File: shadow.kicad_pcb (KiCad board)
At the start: 2 copper layers, 69.8 x 78.7 mm, 100 parts, among them IC2 XB8089D, J1 USB_C_Receptacle, SW1 SW_Push, SW2 SW_Push, SW3 SW_SPST, U1 TCA9548APWR, U2 TCA9548APWR, U3 BQ24092DGQR, U4 TPS61085DGKR, U5 TPS259621DDAT

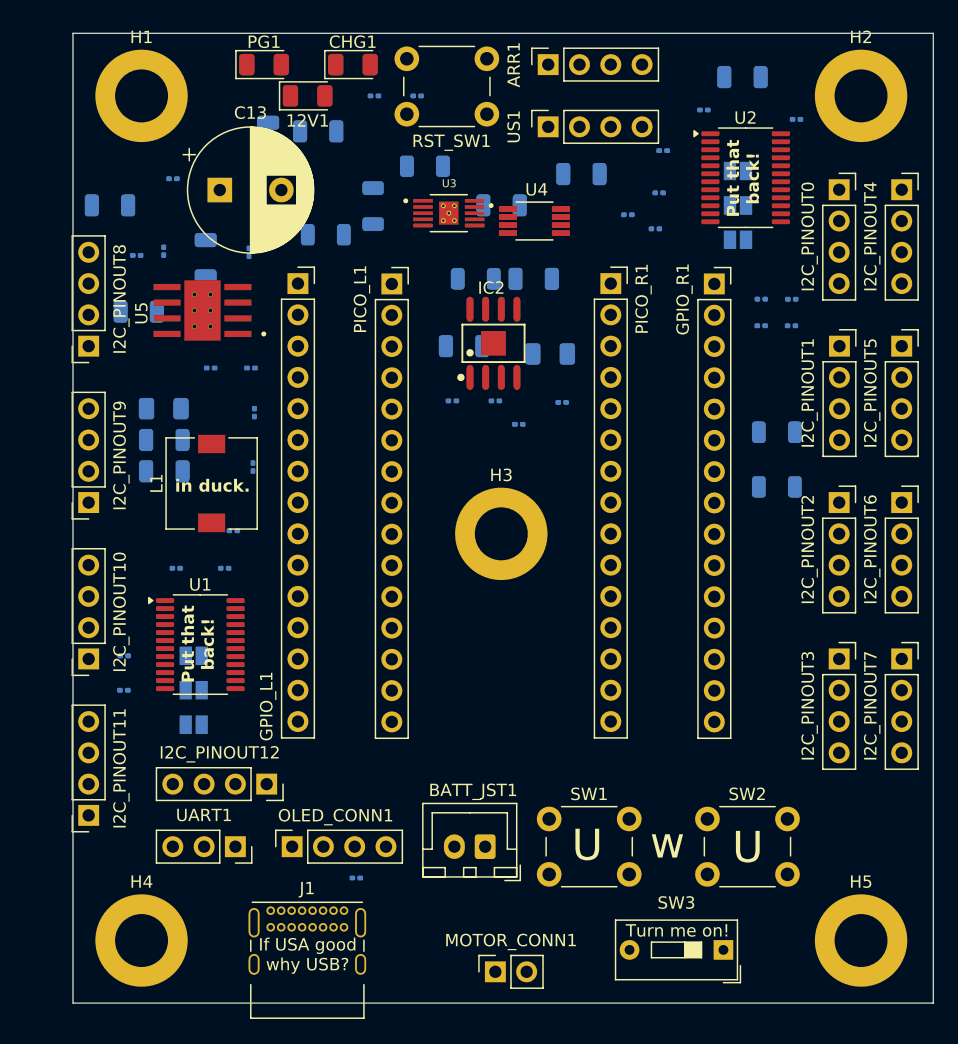
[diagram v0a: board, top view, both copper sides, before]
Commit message: fix some stuff and retrace
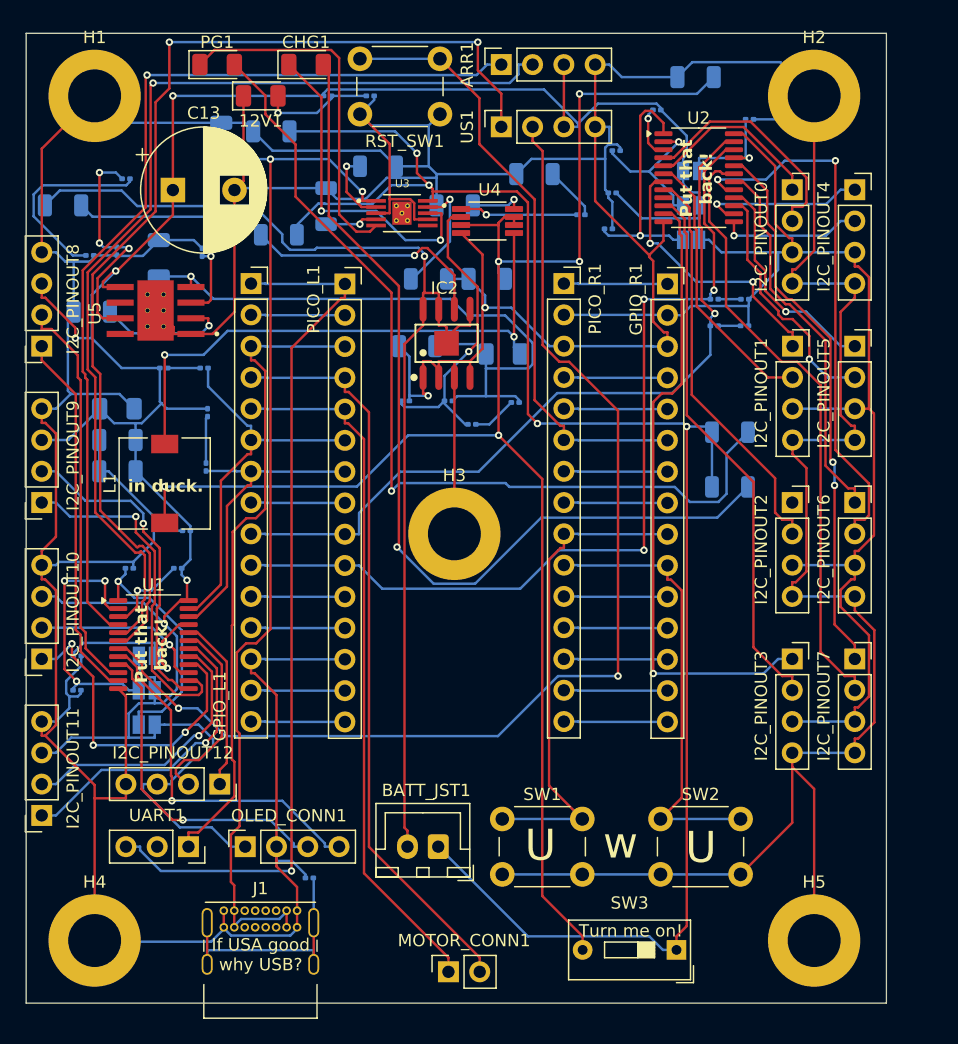
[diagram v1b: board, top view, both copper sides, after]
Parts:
- moved R3 3.81 mm to (125.6, 78.1)
- moved 12V1 3.81 mm to (113.8, 53.3)
- moved ARR1 3.81 mm to (133.3, 50.8)
- moved BATT_JST1 3.81 mm to (128.2, 114.3)
- moved C1 3.81 mm to (136.0, 59.7)
- moved C10 3.81 mm to (100.1, 70.9)
- moved C11 3.81 mm to (102.2, 81.3)
- moved C12 3.81 mm to (102.2, 83.8)
- moved C14 3.81 mm to (107.8, 88.6)
- moved C15 3.81 mm to (142.4, 61.2)
- moved C2 3.81 mm to (129.6, 62.2)
- moved C4 3.81 mm to (126.5, 73.7)
- moved C5 3.81 mm to (149.1, 51.8)
- moved C7 3.81 mm to (97.8, 62.2)
- moved C8 3.81 mm to (110.6, 57.0)
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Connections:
- GPIO_R1 pad 1: /GPIO29 -> /GPIO15
- GPIO_R1 pad 10: /GPIO20 -> /GPIO24
- GPIO_R1 pad 11: /GPIO19 -> /GPIO25
- GPIO_R1 pad 12: /GPIO18 -> /GPIO26
- GPIO_R1 pad 13: GND -> /GPIO27
- GPIO_R1 pad 14: VCC -> /GPIO28
- GPIO_R1 pad 15: /GPIO15 -> /GPIO29
- GPIO_R1 pad 2: /GPIO28 -> VCC
- GPIO_R1 pad 3: /GPIO27 -> GND
- GPIO_R1 pad 4: /GPIO26 -> /GPIO18
- GPIO_R1 pad 5: /GPIO25 -> /GPIO19
- GPIO_R1 pad 6: /GPIO24 -> /GPIO20
- GPIO_R1 pad 7: /GPIO23 -> /GPIO21
- GPIO_R1 pad 9: /GPIO21 -> /GPIO23
- PICO_R1 pad 1: /GPIO29 -> /GPIO15
- PICO_R1 pad 10: /GPIO20 -> /GPIO24
- PICO_R1 pad 11: /GPIO19 -> /GPIO25
- PICO_R1 pad 12: /GPIO18 -> /GPIO26
- PICO_R1 pad 13: GND -> /GPIO27
- PICO_R1 pad 14: VCC -> /GPIO28
- PICO_R1 pad 15: /GPIO15 -> /GPIO29
- PICO_R1 pad 2: /GPIO28 -> VCC
- PICO_R1 pad 3: /GPIO27 -> GND
- PICO_R1 pad 4: /GPIO26 -> /GPIO18
- PICO_R1 pad 5: /GPIO25 -> /GPIO19
- PICO_R1 pad 6: /GPIO24 -> /GPIO20
- PICO_R1 pad 7: /GPIO23 -> /GPIO21
- PICO_R1 pad 9: /GPIO21 -> /GPIO23
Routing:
- net GND: track 0.00 -> 565.2 mm, vias 0 -> 2
- net VCC: track 0.00 -> 315.7 mm, vias 0 -> 5
- net /battery/BAT+: track 0.00 -> 139.7 mm, vias 0 -> 4
- net Net-(SW3-B): track 0.00 -> 132.1 mm, vias 0 -> 5
- net /US_SCL: track 0.00 -> 93.8 mm, vias 0 -> 2
- net /battery/BAT-: track 0.00 -> 92.4 mm, vias 0 -> 1
- net /US_SDA: track 0.00 -> 87.7 mm, vias 0 -> 2
- net Net-(U3-IN): track 0.00 -> 85.2 mm, vias 0 -> 2
- net /SENSOR_SCL: track 0.00 -> 82.4 mm, vias 0 -> 1
- net /SENSOR_SDA: track 0.00 -> 77.5 mm, vias 0 -> 1
- net Net-(CHG1-A): track 0.00 -> 74.8 mm, vias 0 -> 1
- net Net-(PG1-A): track 0.00 -> 74.0 mm, vias 0 -> 1
- net /GPIO9: track 0.00 -> 73.7 mm, vias 0 -> 3
- net /GPIO0: track 0.00 -> 71.7 mm, vias 0 -> 1
- net /GPIO8: track 0.00 -> 63.9 mm, vias 0 -> 1
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
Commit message: v0.0.1
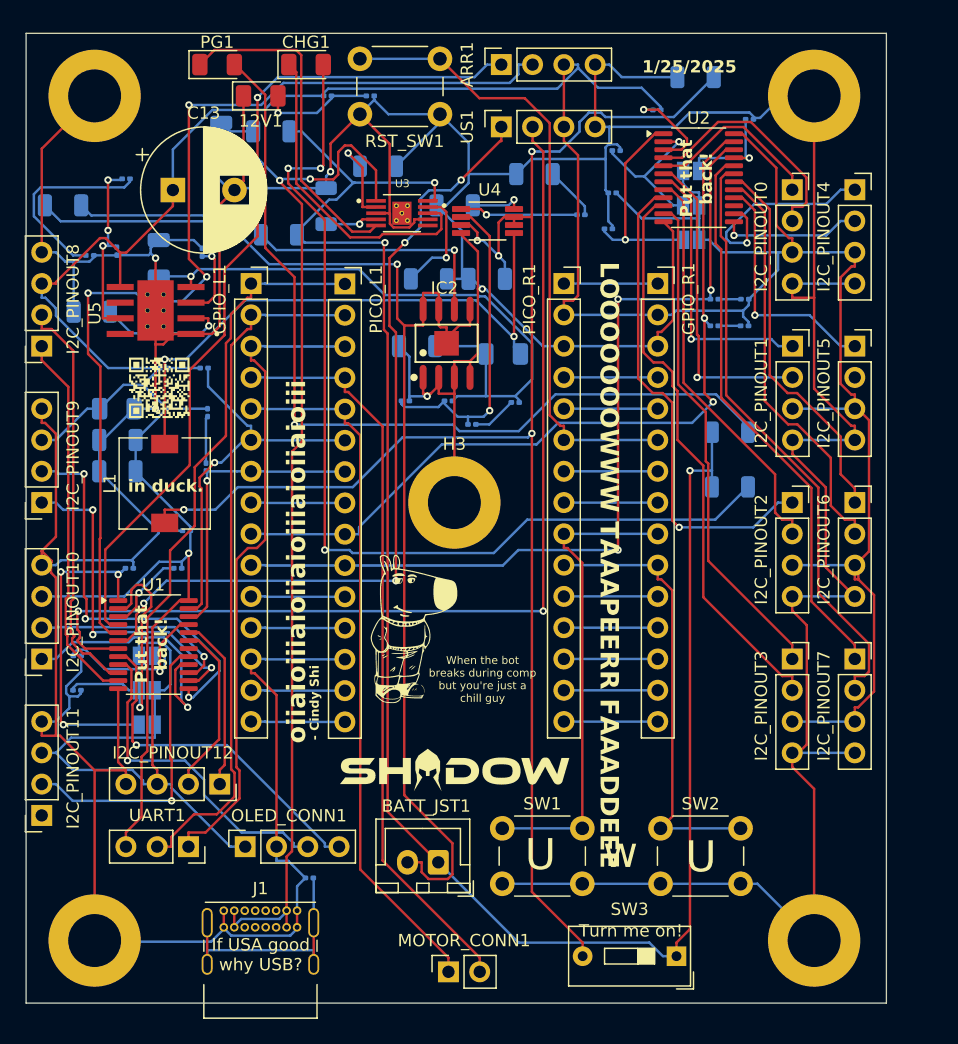
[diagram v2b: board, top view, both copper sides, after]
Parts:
- added G***: LOGO, LOGO, F.Cu at (127.0, 96.5)
- moved H3 2.54 mm to (129.5, 86.4)
- moved BATT_JST1 1.27 mm to (128.2, 115.6)
- moved GPIO_R1 0.79 mm to (146.1, 68.6)
- moved SW1 0.76 mm to (133.4, 112.8)
- moved SW2 0.76 mm to (146.3, 112.8)
- moved SW3 0.51 mm to (147.6, 123.2)
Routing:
- net /GPIO1: track 7.63 -> 56.1 mm
- net /I2C_PINOUT2/SCL: track 0.00 -> 39.9 mm, vias 0 -> 1
- net GND: track 565.2 -> 535.6 mm, vias 2 -> 5
- net /I2C_PINOUT11/SCL: track 25.1 -> 0.00 mm, vias 1 -> 0
- net /US_SDA: track 87.7 -> 67.5 mm, vias 2 -> 4
- net /I2C_PINOUT5/SDA: track 20.1 -> 0.00 mm, vias 1 -> 0
- net VCC: track 315.7 -> 330.3 mm, vias 5 -> 1
- net /GPIO0: track 71.7 -> 57.7 mm, vias 1 -> 0
- net /I2C_PINOUT6/SDA: track 44.3 -> 33.3 mm, vias 2 -> 0
- net /I2C_PINOUT3/SCL: track 51.6 -> 40.9 mm, vias 1 -> 0
- net /battery/BAT+: track 139.7 -> 150.1 mm, vias 4 -> 3
- net /US_SCL: track 93.8 -> 83.6 mm
- net /battery/BAT-: track 92.4 -> 100.6 mm
- net /SENSOR_SDA: track 77.5 -> 69.6 mm
- net /I2C_PINOUT9/SDA: track 26.1 -> 32.6 mm, vias 1 -> 3
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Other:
- board text added: "- Cindy Shi"
- board text added: "1/25/2025"
- board text added: "Designed & Developed by: Evan Yu Logo & Backseating: Aaron Huang"
- board text added: "LOOOOOOOWWW TAAAPEERR FAAADDEEE"
- board text added: "When the bot breaks during comp but you're just a chill guy"
- board text added: "oiiaioiiiaioiiaioiiiaioiiaioiii"
- board text added: "v0.0.1 ymci.ca/shadow"

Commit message: finish pcb
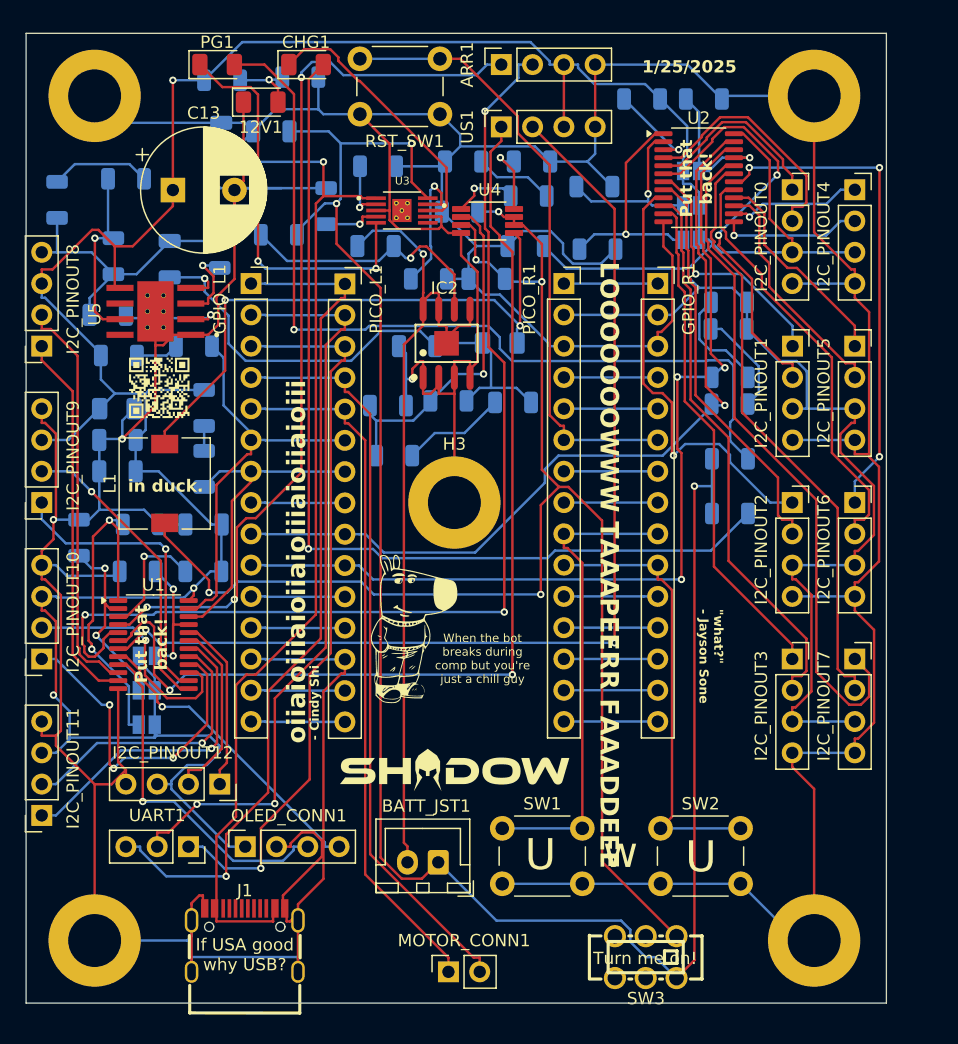
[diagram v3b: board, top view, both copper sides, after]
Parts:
- removed R30: 0k, Resistor_SMD:R_0201_0603Metric
- C14, C15: footprint Capacitor_SMD:C_0201_0603Metric -> Capacitor_SMD:C_1206_3216Metric
- J1: footprint Connector_USB:USB_C_Receptacle_GCT_USB4085 -> USB_C:TYPE-C-SMD_20009-UCAF001-X
- R1, R11, R12, R13, R14, R15, R16, R17, R18, R19, R2, R20, R21, R22, R23, R24, R25, R26, R27, R28, R29, R3, R31, R32, R33, R34, R4: footprint Resistor_SMD:R_0201_0603Metric -> Resistor_SMD:R_1206_3216Metric
- SW3: value SW_SPST -> ~; footprint Button_Switch_THT:SW_DIP_SPSTx01_Slide_9.78x4.72mm_W7.62mm_P2.54mm -> Switch:SW-TH_K3-2235D-F1
- moved C7 25.6 mm to (123.1, 65.5)
- moved C5 22.0 mm to (130.0, 62.7)
- moved R21 12.4 mm to (99.1, 89.2), turned to -90 degrees
- moved R14 8.65 mm to (110.7, 52.1)
- moved R22 8.43 mm to (103.8, 91.9), turned to 0 degrees
- moved C15 8.24 mm to (135.3, 65.5)
- moved C2 7.21 mm to (135.8, 58.7), turned to 0 degrees
- moved R1 6.80 mm to (124.7, 82.5)
- moved R32 6.48 mm to (151.9, 78.4)
- moved R34 6.48 mm to (151.9, 76.2)
- moved C1 5.88 mm to (130.3, 58.7)
- moved R15 5.88 mm to (117.0, 51.8)
- moved R13 5.23 mm to (97.3, 61.8), turned to 90 degrees
- moved R4 4.51 mm to (135.6, 61.5)
- moved R29 4.06 mm to (149.8, 53.6)
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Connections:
- net Net-(U3-IN) renamed VBUS
- C5 pad 1: Net-(SW3-B) -> Net-(U4-EN)
- C6 pad 1: Net-(SW3-B) -> Net-(U4-EN)
- L1 pad 1: Net-(SW3-B) -> Net-(U4-EN)
- SW3 pad 2: Net-(SW3-B) -> unconnected-(SW3-Pad2)
- U4 pad 3: Net-(SW3-B) -> Net-(U4-EN)
- U4 pad 6: Net-(SW3-B) -> Net-(U4-EN)
- U4 pad 7: Net-(SW3-B) -> Net-(U4-EN)
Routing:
- net Net-(SW3-B): track 131.3 -> 0.00 mm, vias 5 -> 0
- net Net-(U4-EN): track 0.00 -> 121.9 mm, vias 0 -> 5
- net GND: track 535.6 -> 571.7 mm, vias 5 -> 3
- net /battery/BAT-: track 100.6 -> 66.6 mm
- net /I2C_PINOUT11/SCL: track 0.00 -> 25.7 mm, vias 0 -> 1
- net Net-(J1-SHIELD): track 21.4 -> 0.00 mm
- net /I2C_PINOUT5/SDA: track 0.00 -> 19.2 mm
- net /US_SDA: track 67.5 -> 83.4 mm, vias 4 -> 2
- net Net-(IC2-VDD): track 36.6 -> 21.8 mm
- net VCC: track 330.3 -> 318.8 mm, vias 1 -> 3
- net /GPIO0: track 57.7 -> 69.2 mm, vias 0 -> 1
- net /I2C_PINOUT6/SCL: track 31.0 -> 40.6 mm, vias 0 -> 3
- net /I2C_PINOUT7/SCL: track 45.8 -> 55.3 mm
- net /I2C_PINOUT1/SDA: track 25.9 -> 34.7 mm, vias 1 -> 2
- net Net-(D1-K): track 52.5 -> 44.2 mm
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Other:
- board text added: "{dblquote}what?{dblquote} - Jayson Sone"
